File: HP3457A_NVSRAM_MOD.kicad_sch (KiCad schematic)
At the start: 15 parts, among them J1 Conn_01x02, U1 TL431DBZ, U10 TC5564APL_Adapter, U2 74AHC2G00, U3 STK12C68

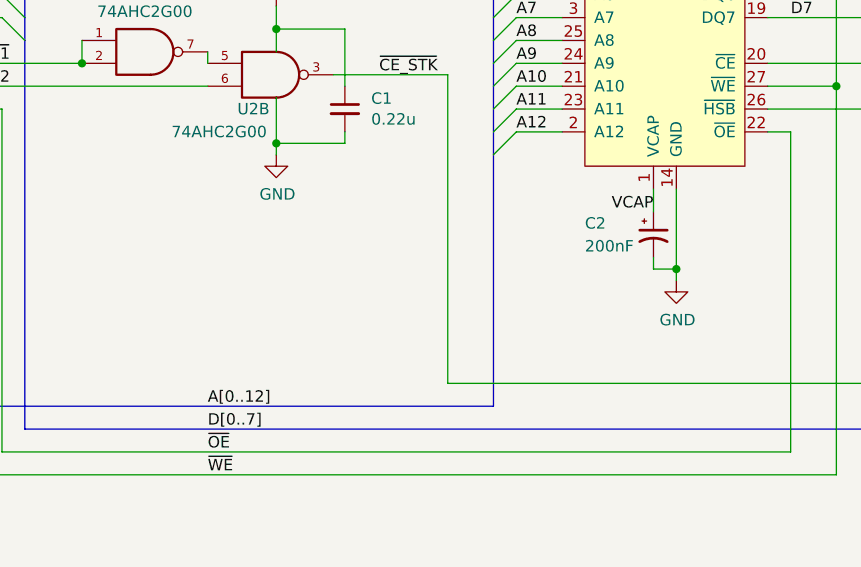
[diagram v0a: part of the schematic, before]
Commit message: Version submitted to OSHPark as V1
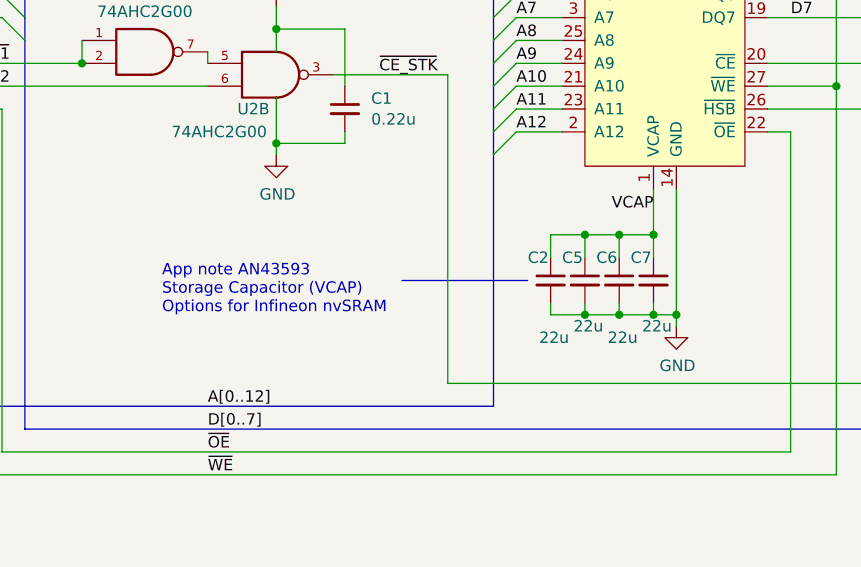
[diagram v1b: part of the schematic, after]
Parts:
- removed C2: 200nF, Capacitor_Tantalum_SMD:CP_EIA-6032-28_Kemet-C, symbol Device:C_Polarized_Small_US
- added C2, C5, C6, C7: 22u, Capacitor_SMD:C_0603_1608Metric, symbol Device:C_Small
- C1, C3, C4: Digikey 311-1087-1-ND -> 1276-1111-2-ND
- J1: MPN (none) -> XX62 nvSRAM V1
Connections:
- net GND: now also C2.2, C5.2, C6.2, C7.2
- net VCAP: now also C2.1, C5.1, C6.1, C7.1
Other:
- note added: "App note AN43593 Storage Capacitor (VCAP) Options for Infineon nvSRAM"
